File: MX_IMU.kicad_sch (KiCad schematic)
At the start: 34 parts, among them SW1 SW_SPST, U1 ld39150dt33-r, U200 STM32F405RGT6, U4 AT24C256, Y200 16MHz

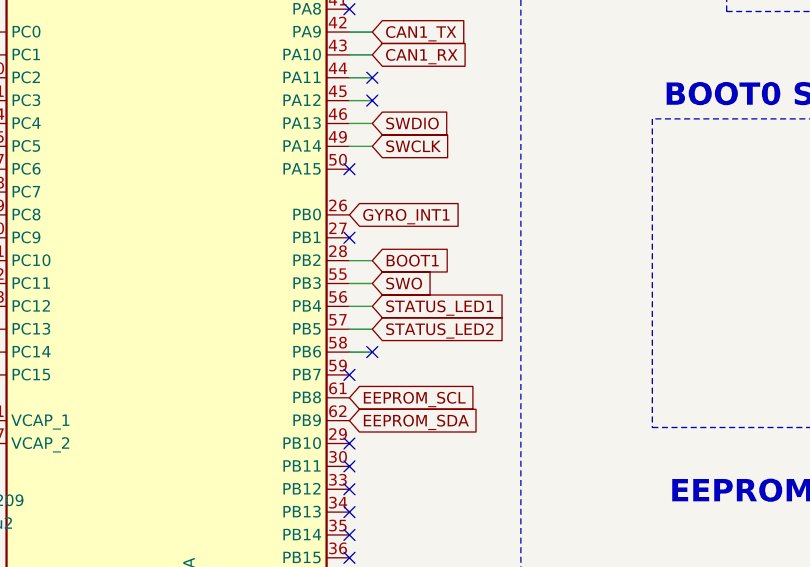
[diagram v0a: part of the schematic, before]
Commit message: Cleanup and check on JCLPCB
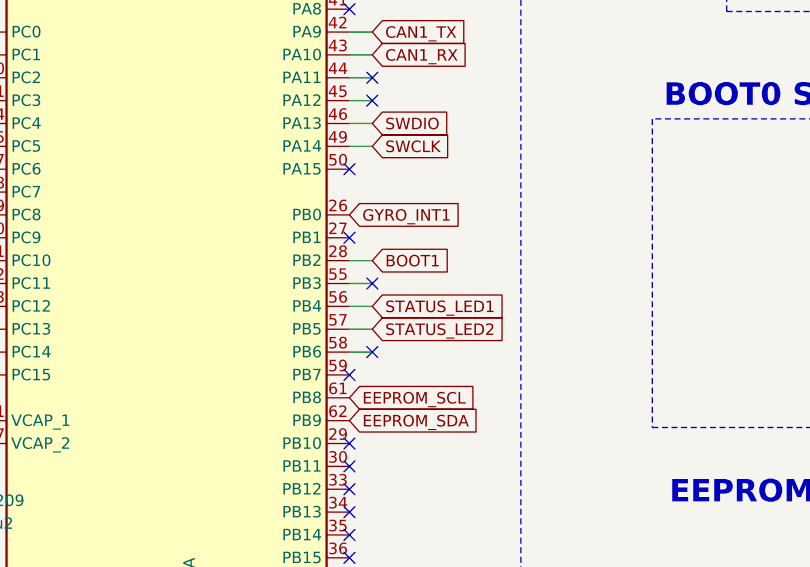
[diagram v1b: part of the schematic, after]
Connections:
- net SWO: no longer names the net of U200.55 (PB3)
- no-connect marks 32 -> 33
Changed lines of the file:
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@@
+	)
+	(no_connect
+		(at 104.14 114.3)
 	)
 	(no_connect
@@
 			(effects
 				(font
-					(size 1.27 1.27)
-				)
-				(hide yes)
-			)
-		)
-	)
-	(global_label "SWO"
-		(shape input)
-		(at 104.14 114.3 0)
-		(effects
-			(font
-				(size 1.27 1.27)
-			)
-			(justify left)
-		)
-		(property "Intersheetrefs" "${INTERSHEET_REFS}"
-			(at 104.14 114.3 0)
-			(effects
-				(font
